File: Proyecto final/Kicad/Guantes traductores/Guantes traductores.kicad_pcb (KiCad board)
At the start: 4 copper layers, 75 x 75 mm, 70 parts, among them J1 USB_C_Receptacle_USB2.0_16P, J10 Contacto1, J11 Contacto2, J12 Contacto3, J13 Contacto4, J3 Flex1, J4 Flex2, J5 Flex3, J6 Flex4, J7 Flex5, SW1 SW_SPST, SW2 SW_SPST, U1 ESP32-C3-WROOM-02, U2 ADS7128IRTER, U3 USBLC6-2SC6, U4 LMV324, U5 LMV324, U6 TPS63020, U7 TP4056 Board, U8 BNO055

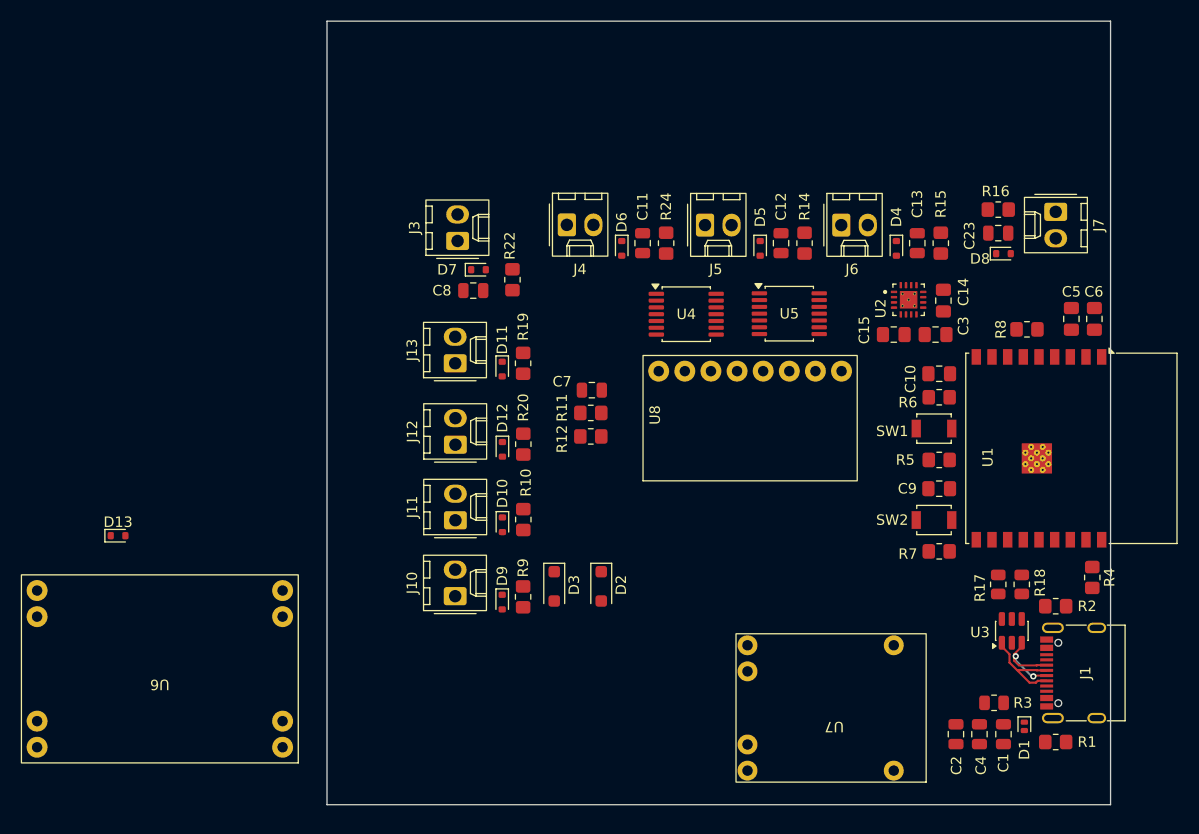
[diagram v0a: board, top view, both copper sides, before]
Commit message: Avance de esquematicos
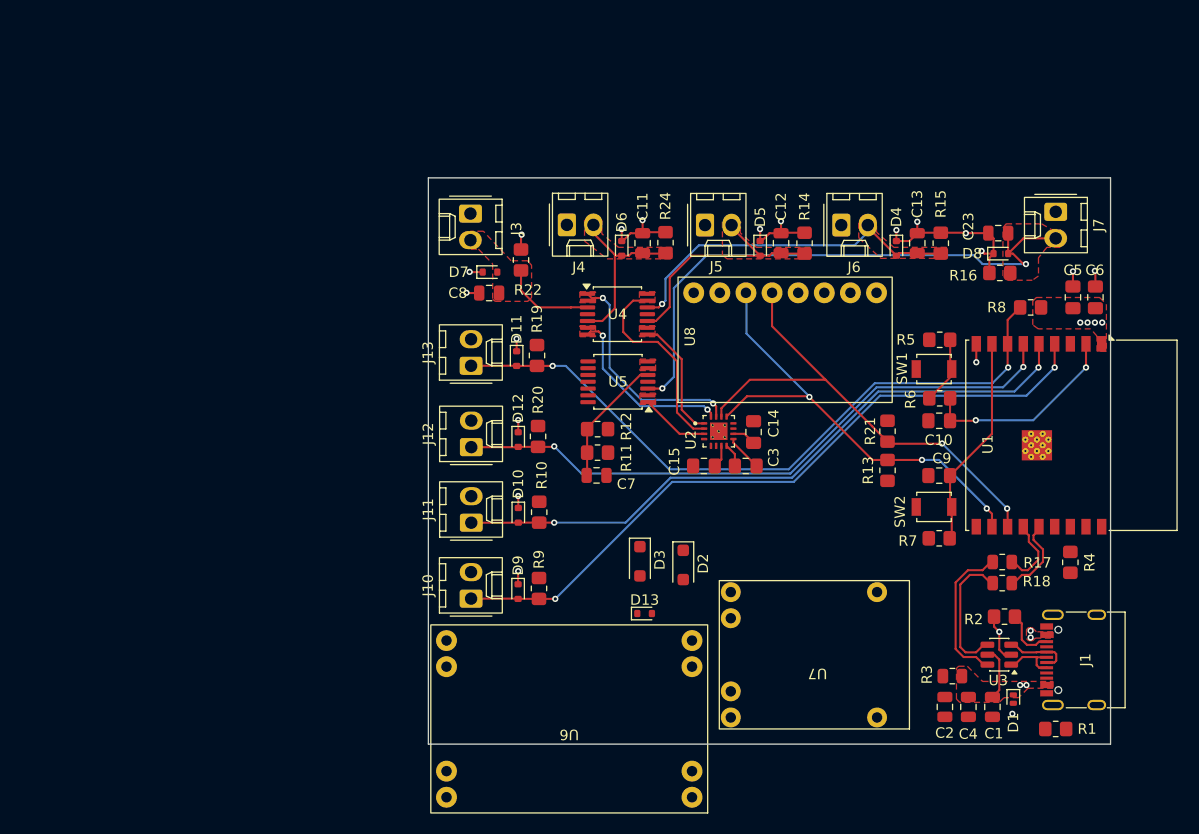
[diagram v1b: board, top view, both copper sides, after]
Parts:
- added R13: 5.1k, Resistor_SMD:R_0805_2012Metric_Pad1.20x1.40mm_HandSolder, F.Cu at (151.4, 155.2)
- added R21: 5.1k, Resistor_SMD:R_0805_2012Metric_Pad1.20x1.40mm_HandSolder, F.Cu at (151.4, 151.5)
- moved D13 50.9 mm to (128.2, 168.9)
- moved U6 39.5 mm to (134.2, 188.0)
- moved C14 22.1 mm to (138.6, 151.6)
- moved C15 22.1 mm to (133.8, 154.8)
- moved C3 22.1 mm to (137.8, 154.8)
- moved U2 22.1 mm to (135.2, 151.5)
- moved U5 17.6 mm to (125.6, 146.8), turned to 180 degrees
- moved R5 11.5 mm to (156.4, 142.8)
- moved D3 8.54 mm to (127.7, 163.9)
- moved U8 8.21 mm to (131.3, 148.8)
- moved C7 8.17 mm to (123.5, 155.7), turned to 180 degrees
- moved D2 8.11 mm to (131.8, 164.3)
- moved U4 6.59 mm to (125.5, 140.3)
- moved R16 6.06 mm to (162.2, 136.3)
- moved SW1 5.70 mm to (155.8, 145.6)
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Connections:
- net Net-(R17-Pad1) renamed /USB-C/R-
- net Net-(R18-Pad1) renamed /USB-C/R+
- U2 pad 18: (no net) -> GND
- U2 pad 19: (no net) -> GND
- U2 pad 20: (no net) -> GND
- U2 pad 21: (no net) -> GND
- U2 pad 22: (no net) -> GND
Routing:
- net IO5: track 0.00 -> 67.3 mm, vias 0 -> 2
- net IO8: track 0.00 -> 65.8 mm, vias 0 -> 2
- net IO6: track 0.00 -> 62.7 mm, vias 0 -> 2
- net IO7: track 0.00 -> 60.4 mm, vias 0 -> 2
- net Net-(J7-Pin_2): track 0.00 -> 56.0 mm, vias 0 -> 2
- net GND: track 0.00 -> 52.2 mm, vias 0 -> 20
- net I2C_SDA: track 0.00 -> 46.6 mm, vias 0 -> 2
- net I2C_SCL: track 0.00 -> 44.7 mm, vias 0 -> 3
- net Net-(J6-Pin_2): track 0.00 -> 34.4 mm, vias 0 -> 1
- net Net-(J5-Pin_2): track 0.00 -> 23.5 mm
- net /Ads7128/AIN0: track 0.00 -> 21.3 mm, vias 0 -> 2
- net IO9: track 0.00 -> 20.4 mm
- net /Esp32 C3 WROOM-02/EN: track 0.00 -> 19.5 mm, vias 0 -> 2
- net /Ads7128/AIN3: track 0.00 -> 19.2 mm
- net /Ads7128/AIN1: track 0.00 -> 17.4 mm, vias 0 -> 2
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- added copper zone on F.Cu, net +3.3V
- added copper zone on In2.Cu, net +3.3V
- added copper zone on F.Cu, net /Ads7128/AIN0
- added copper zone on F.Cu, net /Ads7128/AIN1
- added copper zone on F.Cu, net /Ads7128/AIN2
- added copper zone on F.Cu, net /Ads7128/AIN3
- added copper zone on F.Cu, net /Ads7128/AIN4
- added copper zone on F.Cu, net /Ads7128/AIN5
- added copper zone on In1.Cu, net GND
- added copper zone on F.Cu, net Net-(D1-K)
- added copper zone on In2.Cu, net Net-(D1-K)
- added copper zone on F.Cu, net Net-(J3-Pin_2)
- added copper zone on F.Cu, net Net-(J4-Pin_2)
- added copper zone on F.Cu, net Net-(J5-Pin_2)
- added copper zone on F.Cu, net Net-(J6-Pin_2)
- added copper zone on F.Cu, net Net-(J7-Pin_2)
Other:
- board size 75 x 75 mm -> 65.3 x 54.2 mm
